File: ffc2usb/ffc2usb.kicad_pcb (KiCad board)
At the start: 2 copper layers, 2 parts, among them J1 USB3_A, U1 62674-201121ALF

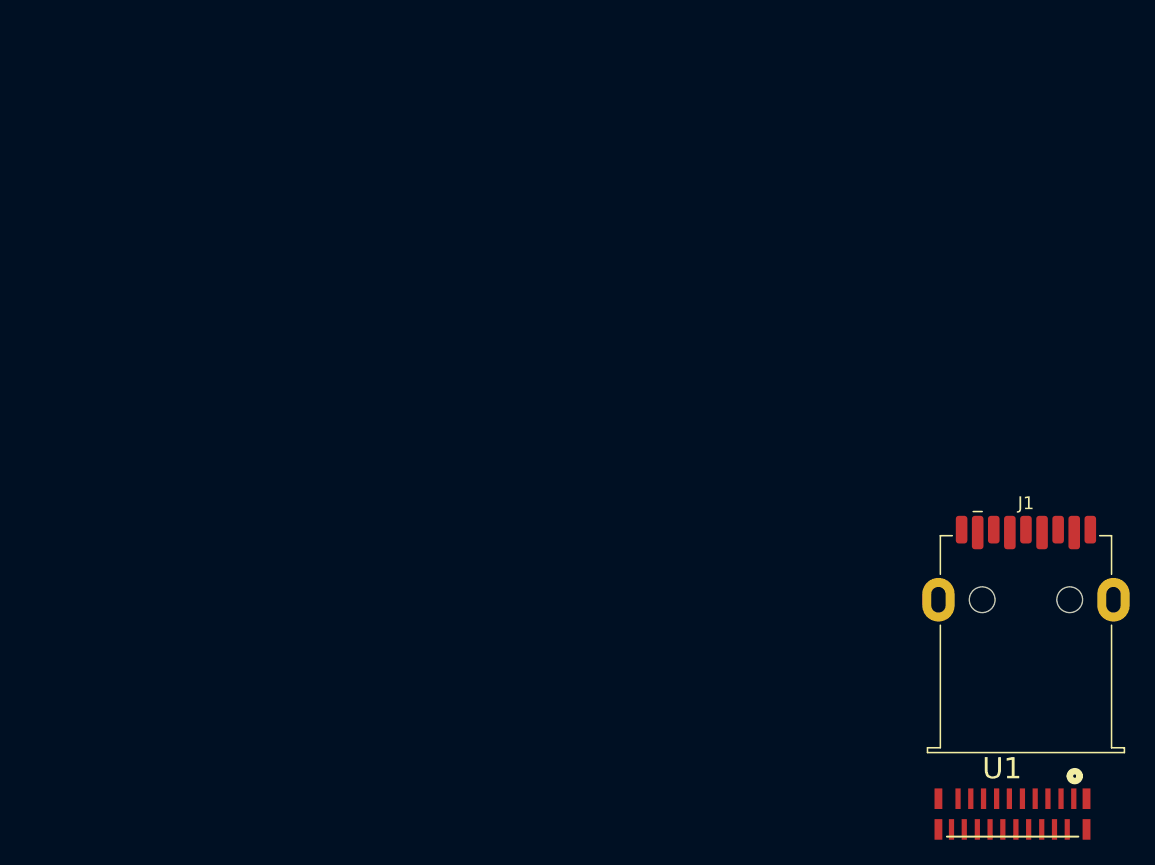
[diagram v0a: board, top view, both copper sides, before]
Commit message: lceda project
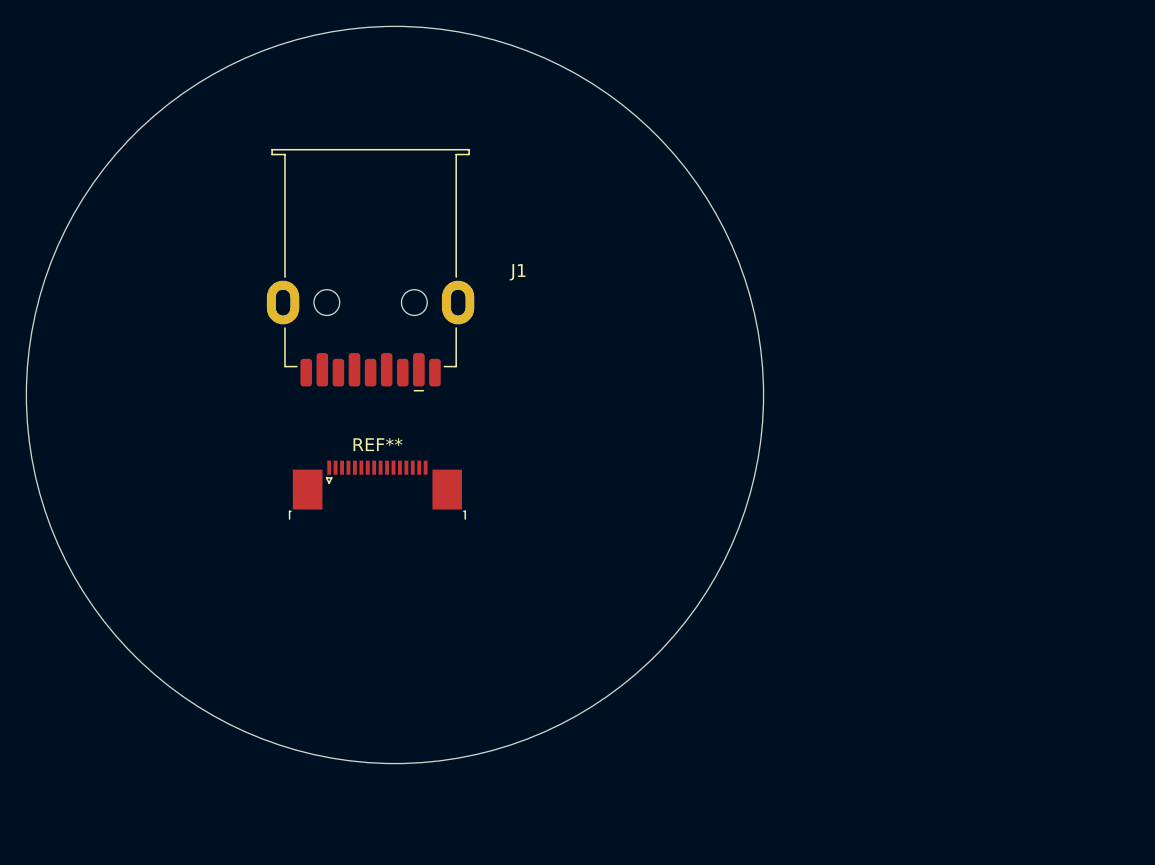
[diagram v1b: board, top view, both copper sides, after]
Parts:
- removed U1: 62674-201121ALF, 62674-201121ALF:FCI_62674-201121ALF
- added REF**: PCB Edge, Connector_FFC-FPC:TE_1-1734839-6_1x16-1MP_P0.5mm_Horizontal, F.Cu at (111.0, 75.0)
- moved J1 59.1 mm to (110.5, 57.4), turned to 180 degrees
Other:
- board outline added: 57.3 x 57.3 mm
